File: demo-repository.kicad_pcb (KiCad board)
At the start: 4 copper layers, 8 x 7.5 mm, 2 parts, among them J1 Screw_Terminal_01x02

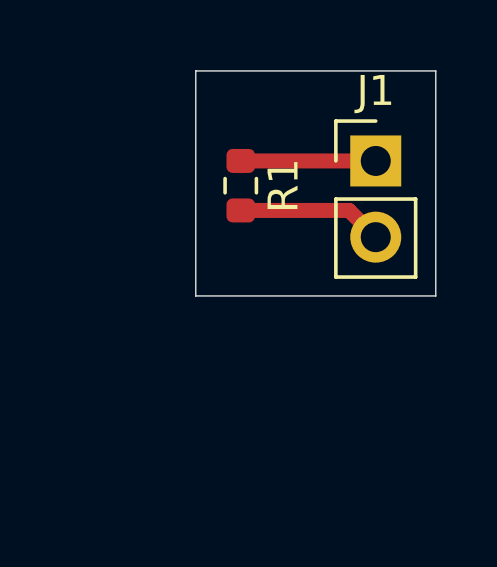
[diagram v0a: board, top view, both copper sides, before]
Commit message: Test for custom DRC checker rules
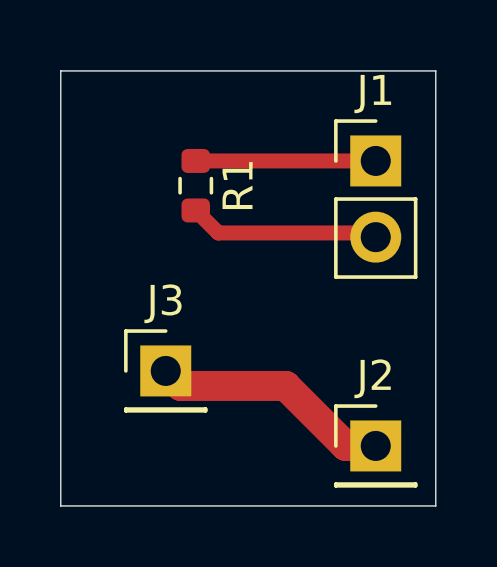
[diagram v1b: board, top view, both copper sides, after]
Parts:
- added J2: Screw_Terminal_01x01, Connector_PinHeader_2.54mm:PinHeader_1x01_P2.54mm_Vertical, F.Cu at (95.5, 68.0)
- added J3: Screw_Terminal_01x01, Connector_PinHeader_2.54mm:PinHeader_1x01_P2.54mm_Vertical, F.Cu at (88.5, 65.5)
- moved R1 1.50 mm to (89.5, 59.3)
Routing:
- net /HV: track 0.00 -> 8.03 mm
- net Net-(J1-Pin_2): track 4.87 -> 6.37 mm
- net Net-(J1-Pin_1): track 4.50 -> 6.00 mm
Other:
- board size 8 x 7.5 mm -> 12.5 x 14.5 mm
